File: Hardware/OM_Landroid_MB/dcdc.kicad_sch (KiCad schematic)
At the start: 23 parts, among them IC3 MAX20405AFOF_VY+T

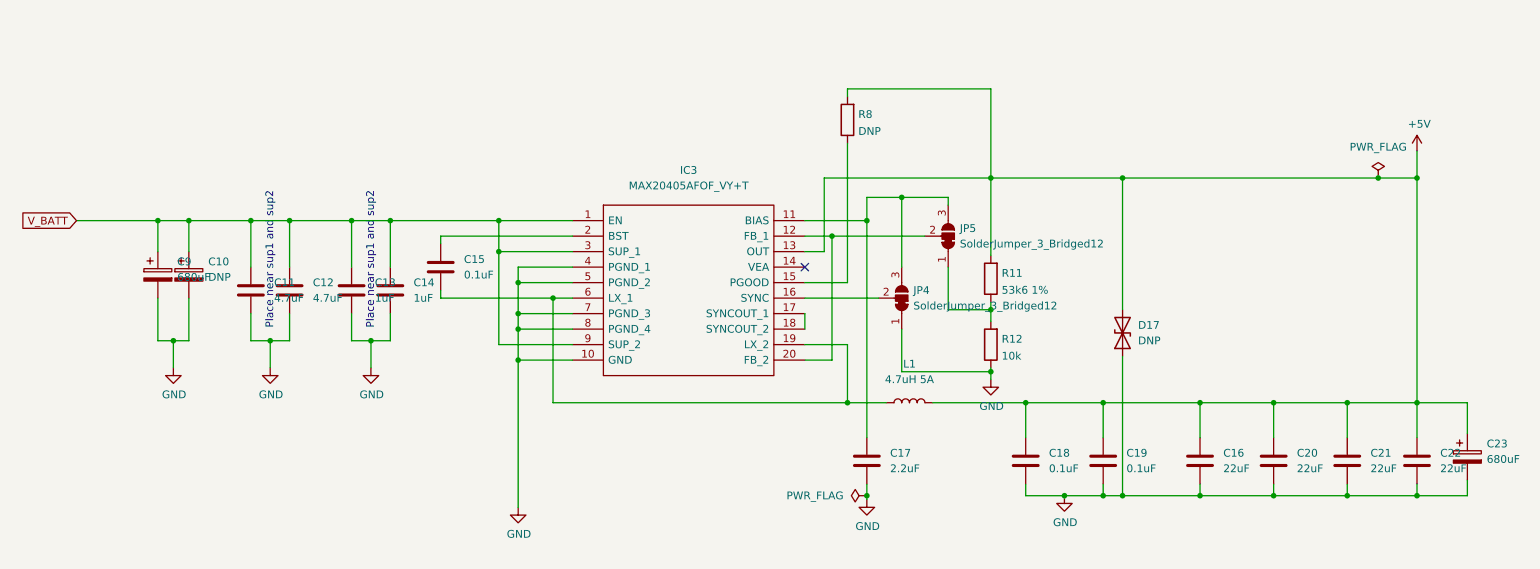
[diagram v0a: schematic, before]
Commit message: Weekend progress
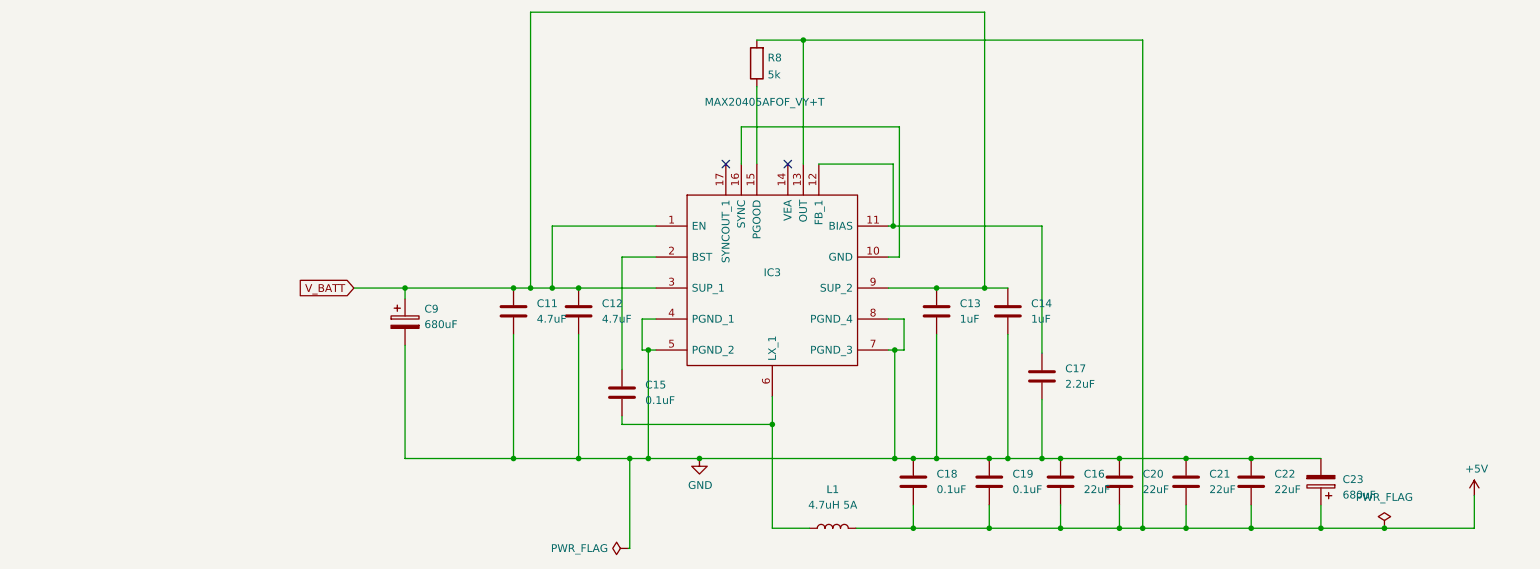
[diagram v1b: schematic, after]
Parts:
- removed C10: DNP, Capacitor_SMD:CP_Elec_10x12.5, symbol Device:C_Polarized
- removed D17: DNP, Diode_SMD:D_0402_1005Metric_Pad0.77x0.64mm_HandSolder, symbol Device:D_TVS
- removed JP4, JP5: SolderJumper_3_Bridged12, Jumper:SolderJumper-3_P1.3mm_Bridged12_Pad1.0x1.5mm, symbol Jumper:SolderJumper_3_Bridged12
- removed R11: 53k6 1%, Resistor_SMD:R_0805_2012Metric_Pad1.20x1.40mm_HandSolder, symbol Device:R
- removed R12: 10k, Resistor_SMD:R_0805_2012Metric_Pad1.20x1.40mm_HandSolder, symbol Device:R
- R8: value DNP -> 5k
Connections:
- net +5V: now also C16.2, C18.2, C19.2, C20.2, C21.2, C22.2; no longer C16.1, C18.1, C19.1, C20.1, C21.1, C22.1
- net GND: now also C16.1, C18.1, C19.1, C20.1, C21.1, C22.1; no longer C16.2, C18.2, C19.2, C20.2, C21.2, C22.2, IC3.10 (GND)
- net at C15.2, IC3.6 (LX_1), L1.1: no longer IC3.19 (LX_2)
- net at IC3.16 (SYNC): now also IC3.10 (GND)
- net at C17.1, IC3.11 (BIAS): now also IC3.12 (FB_1)
- net at IC3.17 (SYNCOUT_1): no longer IC3.18 (SYNCOUT_2)
- no-connect marks 1 -> 2
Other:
- note removed: "Place near sup1 and sup2"
- moved on the sheet: C11, C12, C13, C14, C15, C16, C17, C18, C19, C20, C21, C22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
